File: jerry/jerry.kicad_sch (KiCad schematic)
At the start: 14 parts, among them J1 0532610471, J2 0532610471, J3 0532610471, J4 XT60-M, J7 TSW-106-06-F-S-LL, J8 TSW-106-06-F-S-LL, U1 RASPBERRY_PI_4B_4GB, U2 A4988_STEPPER_MOTOR_DRIVER_CA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

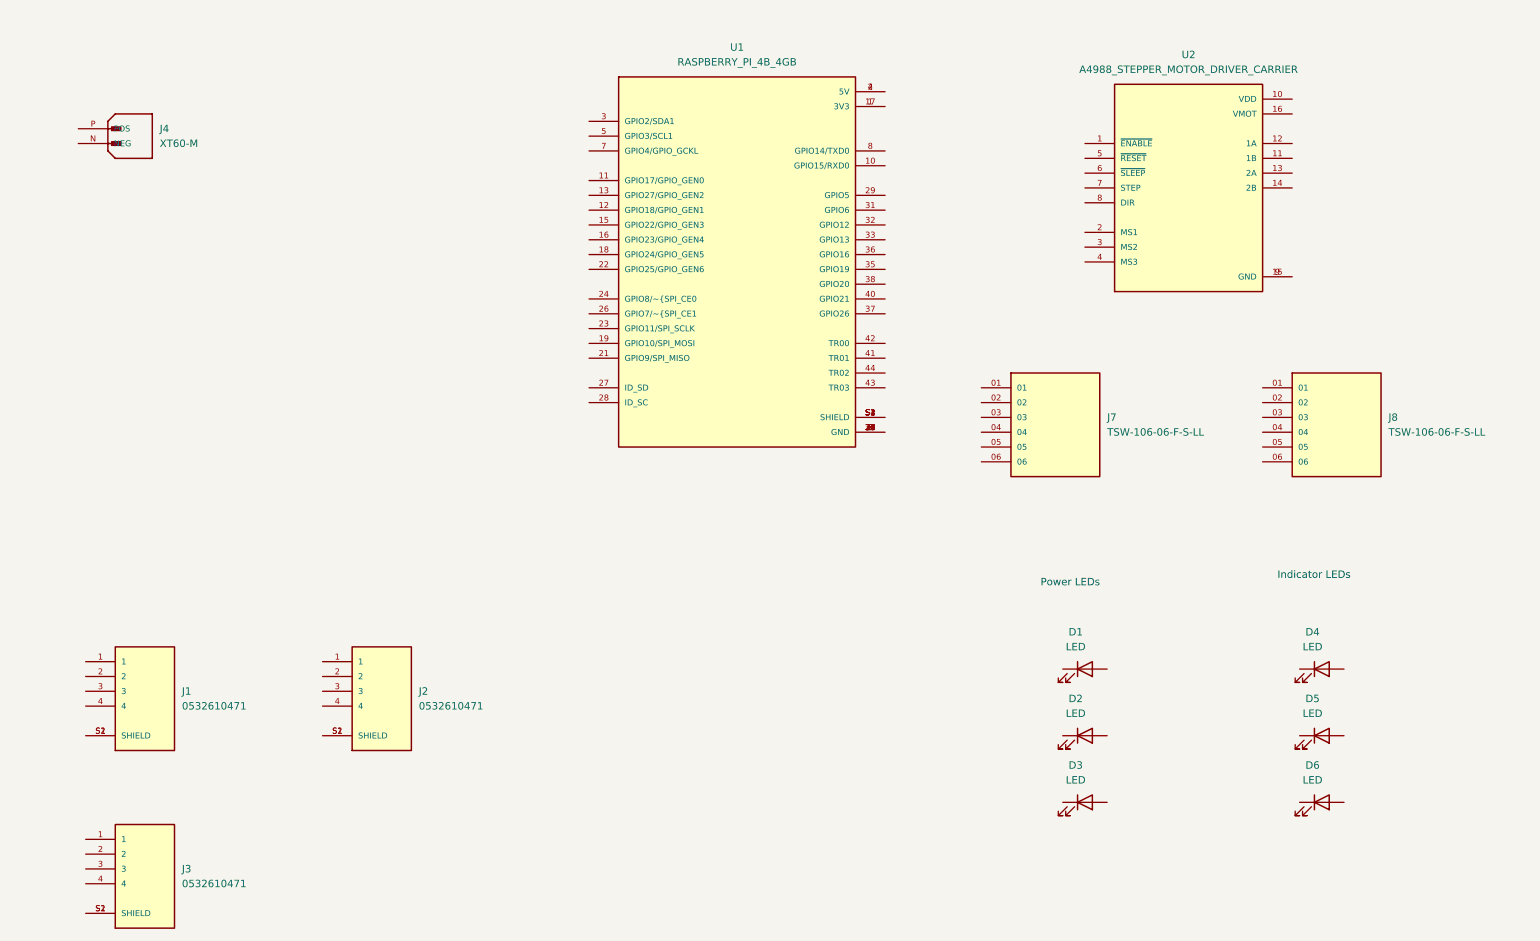
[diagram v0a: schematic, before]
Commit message: some updates
updated schematic, added components
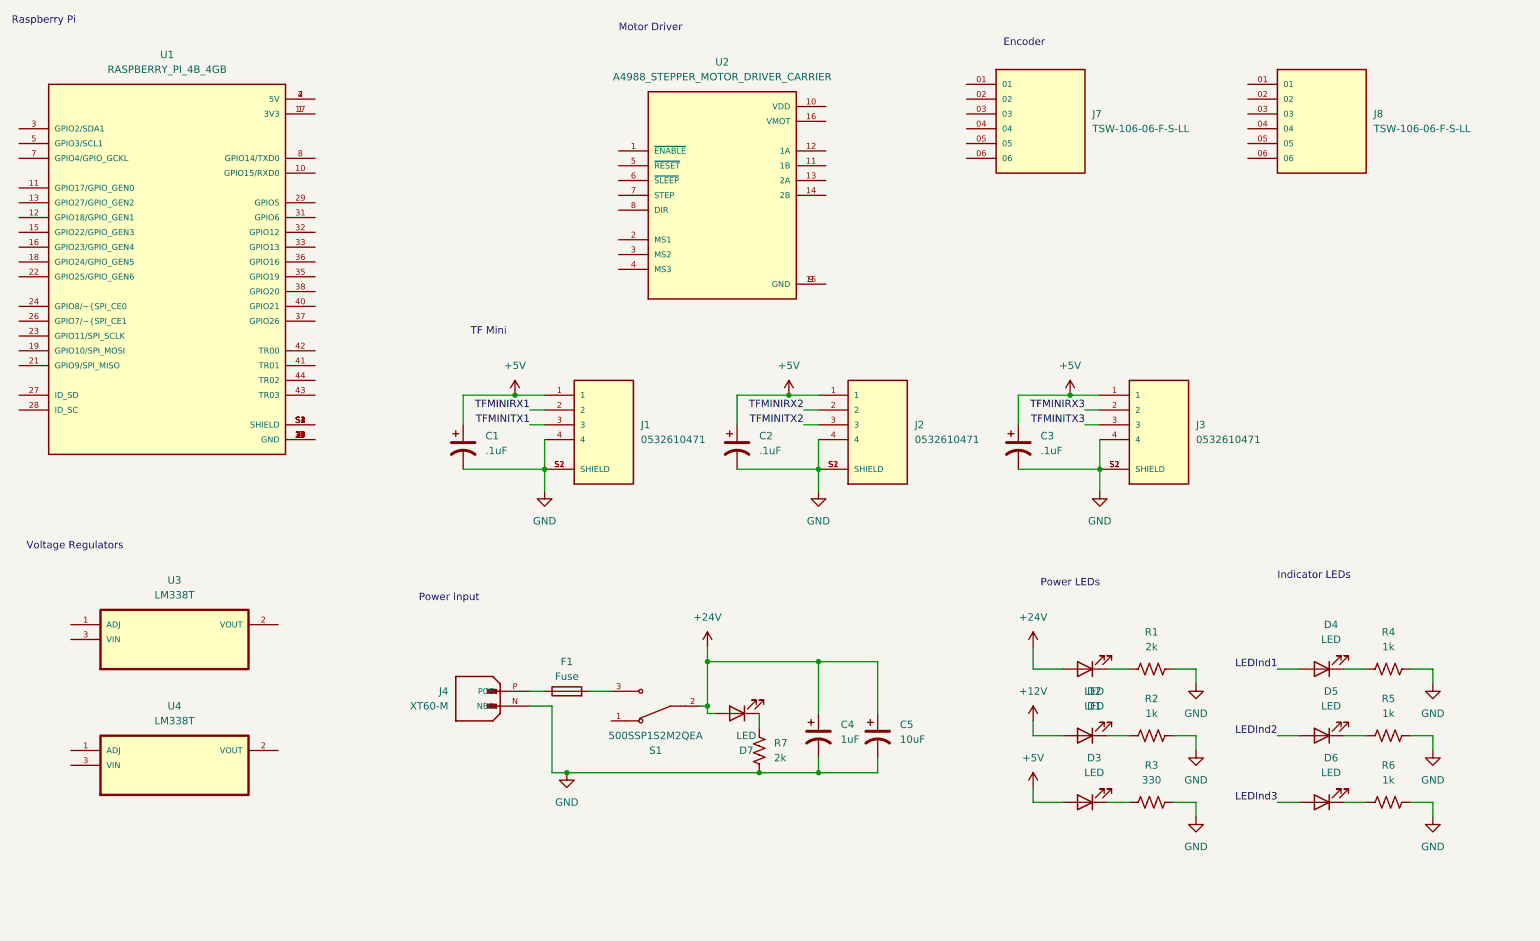
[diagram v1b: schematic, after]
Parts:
- added C1, C2, C3: .1uF, symbol Device:C_Polarized_US
- added C4: 1uF, symbol Device:C_Polarized_US
- added C5: 10uF, symbol Device:C_Polarized_US
- added D7: LED, Diode_SMD:D_0201_0603Metric_Pad0.64x0.40mm_HandSolder, symbol Device:LED
- added F1: Fuse, symbol Device:Fuse
- added R1, R7: 2k, symbol Device:R_US
- added R2, R4, R5, R6: 1k, symbol Device:R_US
- added R3: 330, symbol Device:R_US
- added S1: 500SSP1S2M2QEA, SW_500SSP1S2M2QEA, symbol jerry:500SSP1S2M2QEA
- added U3, U4: LM338T, jerry:TO254P1054X470X1955-3, symbol jerry:LM338T
- J1, J2, J3: footprint (none) -> jerry:MOLEX_0532610471
- J4: footprint (none) -> jerry:AMASS_XT60-M
- J7, J8: footprint (none) -> jerry:SAMTEC_TSW-106-06-F-S-LL
- U2: footprint (none) -> jerry:MODULE_A4988_STEPPER_MOTOR_DRIVER_CARRIER
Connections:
- net at D3.1 (K): now also R3.1
- net +5V: now reaches D3.2 (A)
- net +5V: now also J1.1, J2.1, J3.1, C1.1, C2.1, C3.1
- net at D6.1 (K): now also R6.1
- net LEDInd3: now reaches D6.2 (A)
- net TFMINIRX3: now reaches J3.2
- net TFMINITX3: now reaches J3.3
- net GND: now reaches J3.4
- net GND: now also J1.4, J1.S1 (SHIELD), J1.S2 (SHIELD), J2.4, J2.S1 (SHIELD), J2.S2 (SHIELD), J3.S1 (SHIELD), J3.S2 (SHIELD), J4.N (NEG), C1.2, C2.2, C3.2, C4.2, C5.2, R1.2, R2.2, R3.2, R4.2, R5.2, R6.2, R7.1
- net at J4.P (POS): now also F1.1
- net at D4.1 (K): now also R4.1
- net LEDInd1: now reaches D4.2 (A)
- net TFMINIRX1: now reaches J1.2
- net TFMINITX1: now reaches J1.3
- net at D1.1 (K): now also R1.1
- net +24V: now reaches D1.2 (A)
- net +24V: now also C4.1, C5.1, D7.2 (A), S1.2
- net at D2.1 (K): now also R2.1
- net +12V: now reaches D2.2 (A)
- net TFMINIRX2: now reaches J2.2
- net TFMINITX2: now reaches J2.3
- net at D5.1 (K): now also R5.1
- net LEDInd2: now reaches D5.2 (A)
- new net: D7.1 (K), R7.2
- new net: F1.2, S1.3
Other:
- note added: "Encoder"
- note added: "Motor Driver"
- note added: "Power Input"
- note added: "Raspberry Pi"
- note added: "TF Mini"
- note added: "Voltage Regulators"
- moved on the sheet: D1, D2, D3, D4, D5, D6, J1, J2, J3, J4, J7, J8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
